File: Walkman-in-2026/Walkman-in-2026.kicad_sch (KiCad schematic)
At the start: 22 parts, among them J2 Micro_SD_Card, Q1 BSS138, Q2 BSS138, SW1 SW_Push, SW2 SW_Push, SW3 SW_Push, SW4 SW_SPDT, SW5 SW_Push, SW6 SW_Push, U1 XIAO-ESP32-S3-DIP

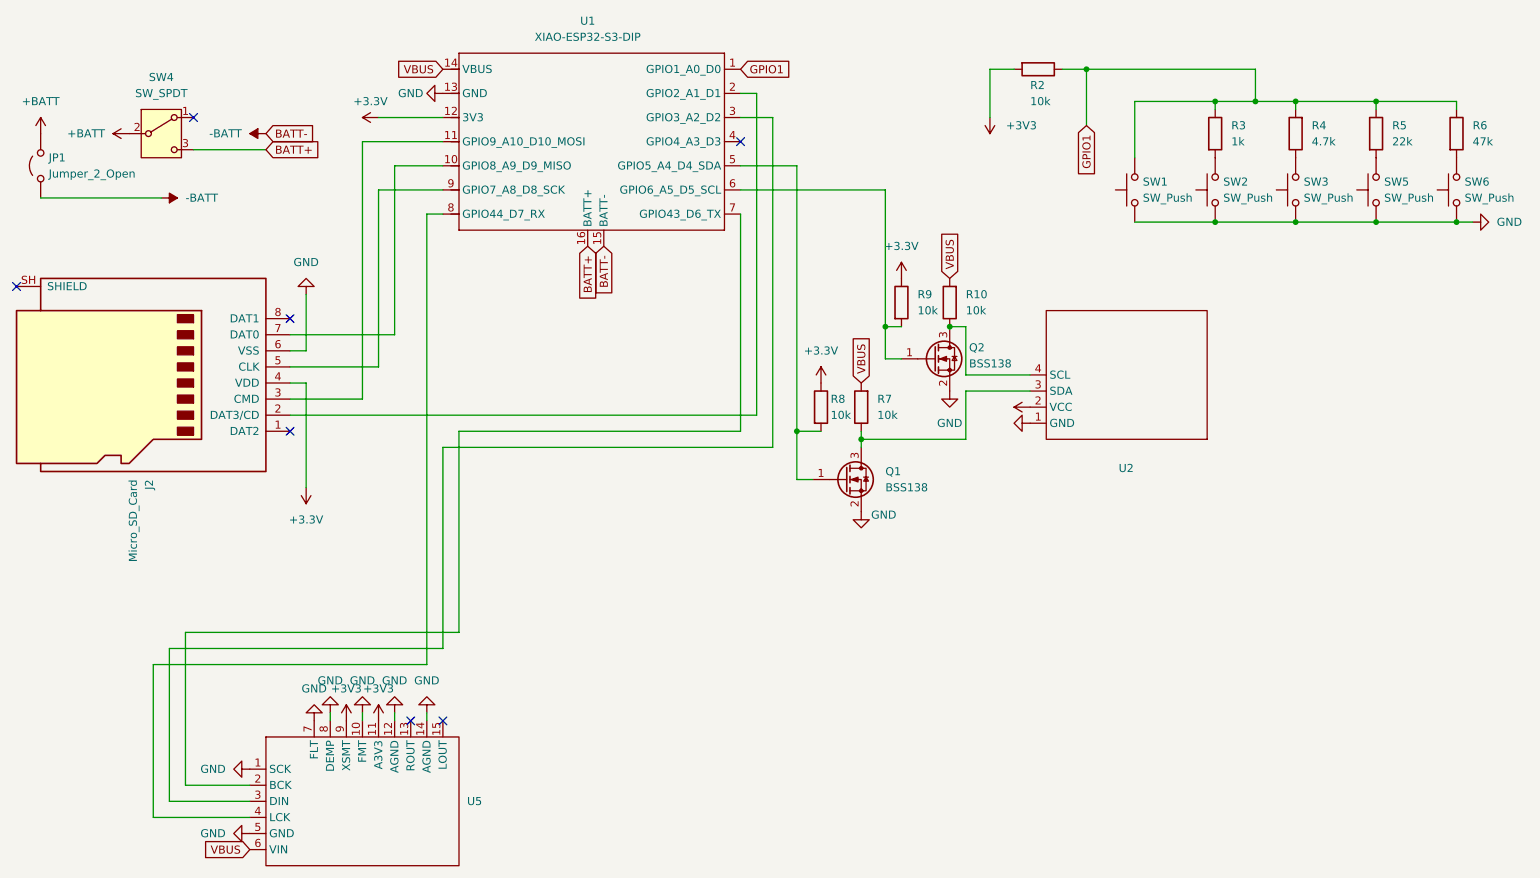
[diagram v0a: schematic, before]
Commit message: v1 final
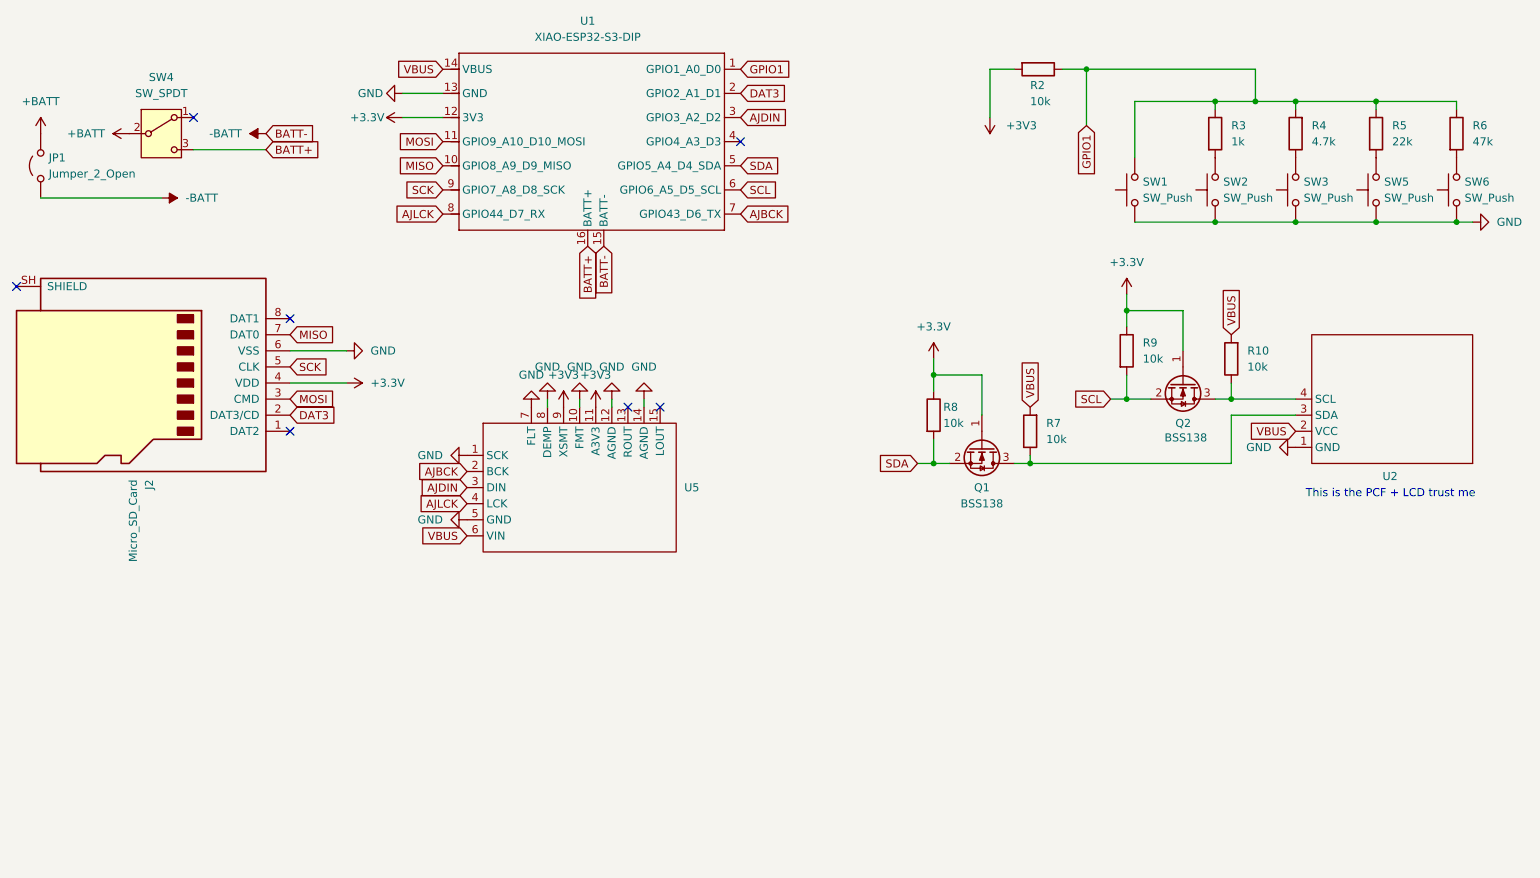
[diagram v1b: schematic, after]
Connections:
- net +5V is gone; now on net VBUS: U2.2 (VCC)
- net +3.3V: now also Q1.1 (G), Q2.1 (G)
- net GND: no longer Q1.2 (S), Q2.2 (S)
- net SCL: now reaches R9.2, U1.6 (GPIO6_A5_D5_SCL)
- net SCL: now also Q2.2 (S); no longer Q2.1 (G)
- net DAT3: now reaches J2.2 (DAT3/CD), U1.2 (GPIO2_A1_D1)
- net MOSI: now reaches J2.3 (CMD), U1.11 (GPIO9_A10_D10_MOSI)
- net SCK: now reaches J2.5 (CLK), U1.9 (GPIO7_A8_D8_SCK)
- net MISO: now reaches J2.7 (DAT0), U1.10 (GPIO8_A9_D9_MISO)
- net SDA: now reaches R8.2, U1.5 (GPIO5_A4_D4_SDA)
- net SDA: now also Q1.2 (S); no longer Q1.1 (G)
- net AJDIN: now reaches U1.3 (GPIO3_A2_D2), U5.3 (DIN)
- net AJBCK: now reaches U1.7 (GPIO43_D6_TX), U5.2 (BCK)
- net AJLCK: now reaches U1.8 (GPIO44_D7_RX), U5.4 (LCK)
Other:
- note added: "This is the PCF + LCD trust me"
- moved on the sheet: Q1, Q2, R10, R7, R8, R9, U2, U5
